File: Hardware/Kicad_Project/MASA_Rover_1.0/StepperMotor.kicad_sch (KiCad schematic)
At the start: 8 parts, among them J26 Conn_01x04_Male, J27 Conn_01x04_Male, J28 Screw_Terminal_01x01, J29 Screw_Terminal_01x01

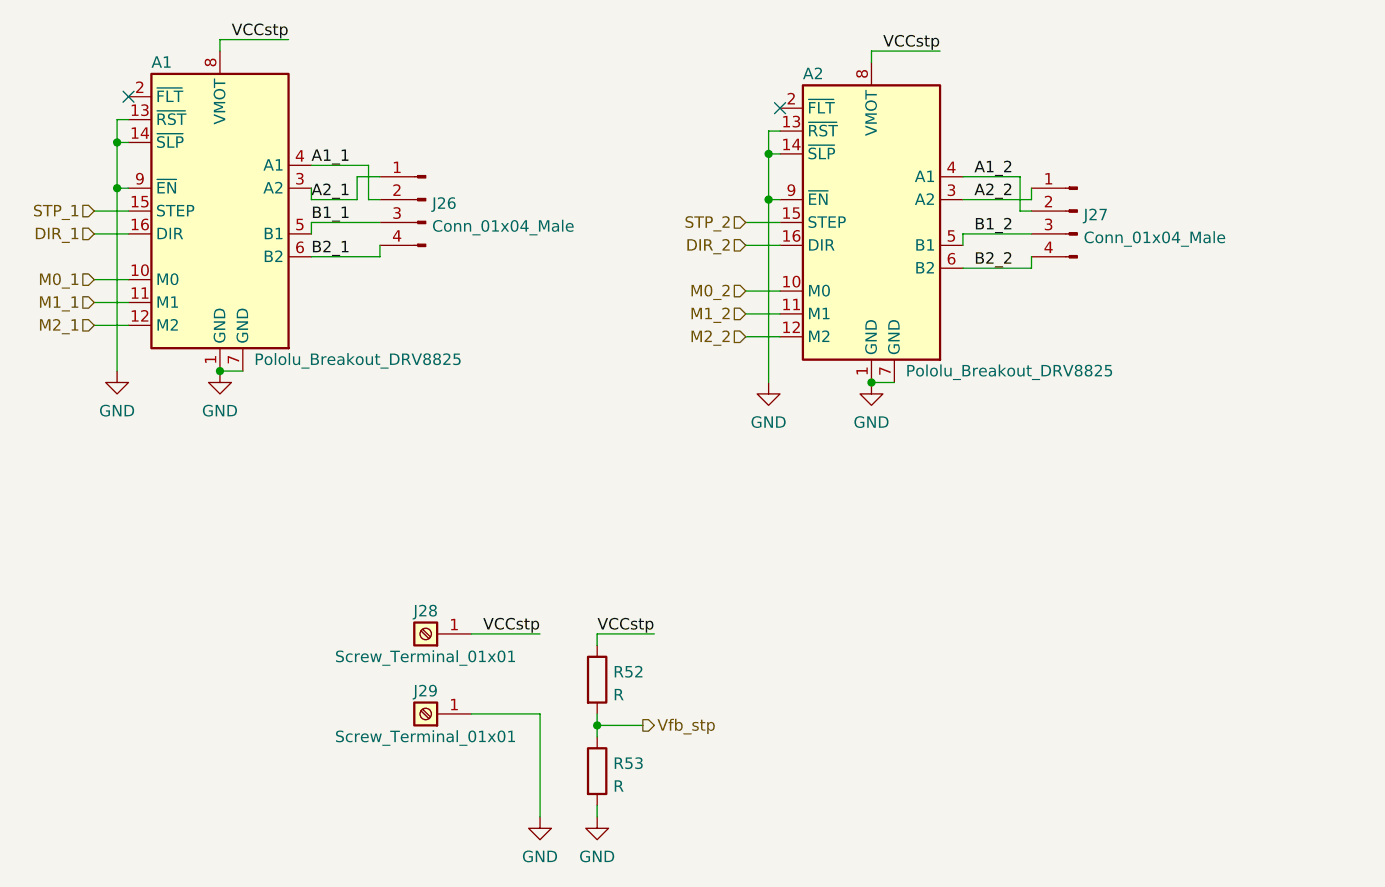
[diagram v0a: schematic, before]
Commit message: update hardware
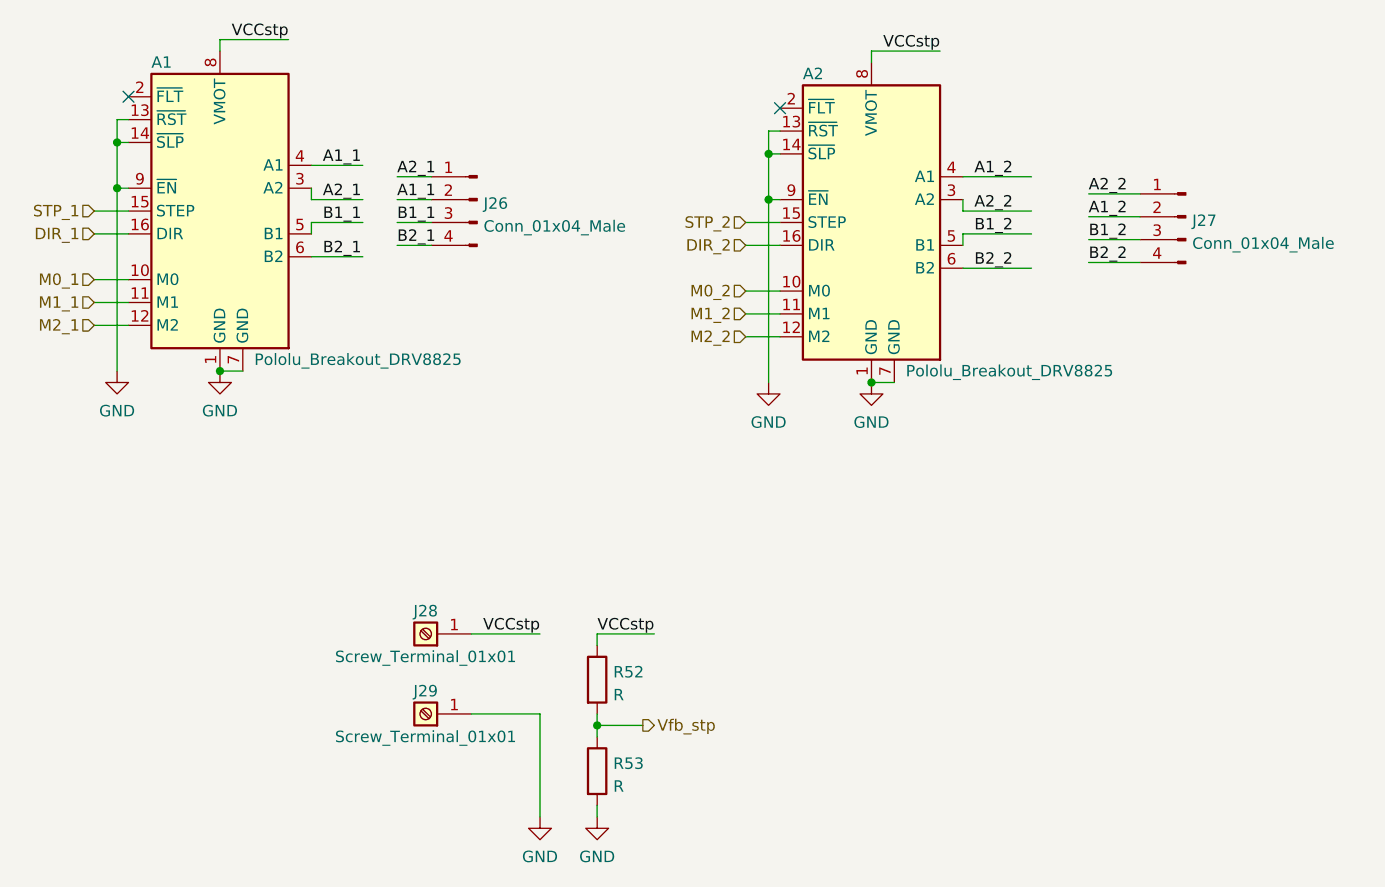
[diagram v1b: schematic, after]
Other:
- moved on the sheet: J26, J27
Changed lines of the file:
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@@
-    (stroke (width 0) (type default) (color 0 0 0 0))
-  )
-  (wire (pts (xy 97.79 81.28) (xy 97.79 85.09))
-    (stroke (width 0) (type default) (color 0 0 0 0))
-  )
-  (wire (pts (xy 96.52 85.09) (xy 96.52 82.55))
     (stroke (width 0) (type default) (color 0 0 0 0))
   )
@@
     (stroke (width 0) (type default) (color 0 0 0 0))
   )
-  (wire (pts (xy 97.79 81.28) (xy 91.44 81.28))
-    (stroke (width 0) (type default) (color 0 0 0 0))
-  )
   (wire (pts (xy 153.67 105.41) (xy 156.21 105.41))
     (stroke (width 0) (type default) (color 0 0 0 0))
@@
     (stroke (width 0) (type default) (color 0 0 0 0))
   )
-  (wire (pts (xy 171.45 92.71) (xy 171.45 91.44))
-    (stroke (width 0) (type default) (color 0 0 0 0))
-  )
-  (wire (pts (xy 97.79 85.09) (xy 99.06 85.09))
+  (wire (pts (xy 91.44 91.44) (xy 97.155 91.44))
+    (stroke (width 0) (type default) (color 0 0 0 0))
+  )
+  (wire (pts (xy 163.83 82.55) (xy 171.45 82.55))
     (stroke (width 0) (type default) (color 0 0 0 0))
   )
@@
     (stroke (width 0) (type default) (color 0 0 0 0))
   )
+  (wire (pts (xy 177.8 89.535) (xy 183.515 89.535))
+    (stroke (width 0) (type default) (color 0 0 0 0))
+  )
   (wire (pts (xy 123.19 142.24) (xy 123.19 143.51))
     (stroke (width 0) (type default) (color 0 0 0 0))
@@
     (stroke (width 0) (type default) (color 0 0 0 0))
   )
+  (wire (pts (xy 91.44 81.28) (xy 97.155 81.28))
+    (stroke (width 0) (type default) (color 0 0 0 0))
+  )
+  (wire (pts (xy 171.45 86.36) (xy 163.83 86.36))
+    (stroke (width 0) (type default) (color 0 0 0 0))
+  )
   (wire (pts (xy 67.31 96.52) (xy 71.12 96.52))
     (stroke (width 0) (type default) (color 0 0 0 0))
@@
     (stroke (width 0) (type default) (color 0 0 0 0))
   )
+  (wire (pts (xy 100.965 85.09) (xy 104.775 85.09))
+    (stroke (width 0) (type default) (color 0 0 0 0))
+  )
   (wire (pts (xy 142.24 80.01) (xy 143.51 80.01))
     (stroke (width 0) (type default) (color 0 0 0 0))
@@
     (stroke (width 0) (type default) (color 0 0 0 0))
   )
-  (wire (pts (xy 96.52 82.55) (xy 99.06 82.55))
-    (stroke (width 0) (type default) (color 0 0 0 0))
-  )
-  (wire (pts (xy 99.06 91.44) (xy 99.06 90.17))
-    (stroke (width 0) (type default) (color 0 0 0 0))
-  )
   (wire (pts (xy 88.9 67.31) (xy 81.28 67.31))
     (stroke (width 0) (type default) (color 0 0 0 0))
@@
     (stroke (width 0) (type default) (color 0 0 0 0))
   )
+  (wire (pts (xy 177.8 84.455) (xy 183.515 84.455))
+    (stroke (width 0) (type default) (color 0 0 0 0))
+  )
   (wire (pts (xy 116.84 142.24) (xy 116.84 153.67))
     (stroke (width 0) (type default) (color 0 0 0 0))
   )
+  (wire (pts (xy 100.965 87.63) (xy 104.775 87.63))
+    (stroke (width 0) (type default) (color 0 0 0 0))
+  )
   (wire (pts (xy 123.19 143.51) (xy 123.19 144.78))
     (stroke (width 0) (type default) (color 0 0 0 0))
   )
-  (wire (pts (xy 91.44 91.44) (xy 99.06 91.44))
-    (stroke (width 0) (type default) (color 0 0 0 0))
-  )
-  (wire (pts (xy 99.06 87.63) (xy 91.44 87.63))
+  (wire (pts (xy 91.44 87.63) (xy 97.155 87.63))
     (stroke (width 0) (type default) (color 0 0 0 0))
   )
@@
     (stroke (width 0) (type default) (color 0 0 0 0))
   )
-  (wire (pts (xy 91.44 85.09) (xy 96.52 85.09))
+  (wire (pts (xy 100.965 90.17) (xy 104.775 90.17))
     (stroke (width 0) (type default) (color 0 0 0 0))
   )
@@
     (stroke (width 0) (type default) (color 0 0 0 0))
   )
+  (wire (pts (xy 91.44 85.09) (xy 97.155 85.09))
+    (stroke (width 0) (type default) (color 0 0 0 0))
+  )
   (wire (pts (xy 142.24 77.47) (xy 143.51 77.47))
     (stroke (width 0) (type default) (color 0 0 0 0))
   )
-  (wire (pts (xy 170.18 86.36) (xy 171.45 86.36))
+  (wire (pts (xy 100.965 82.55) (xy 104.775 82.55))
     (stroke (width 0) (type default) (color 0 0 0 0))
   )
@@
     (stroke (width 0) (type default) (color 0 0 0 0))
   )
-  (wire (pts (xy 163.83 82.55) (xy 170.18 82.55))
-    (stroke (width 0) (type default) (color 0 0 0 0))
-  )
-  (wire (pts (xy 163.83 85.09) (xy 171.45 85.09))
+  (wire (pts (xy 163.83 86.36) (xy 163.83 85.09))
     (stroke (width 0) (type default) (color 0 0 0 0))
   )
@@
     (stroke (width 0) (type default) (color 0 0 0 0))
   )
-  (wire (pts (xy 170.18 82.55) (xy 170.18 86.36))
-    (stroke (width 0) (type default) (color 0 0 0 0))
-  )
-  (wire (pts (xy 171.45 85.09) (xy 171.45 83.82))
+  (wire (pts (xy 177.8 92.075) (xy 183.515 92.075))
+    (stroke (width 0) (type default) (color 0 0 0 0))
+  )
+  (wire (pts (xy 177.8 86.995) (xy 183.515 86.995))
     (stroke (width 0) (type default) (color 0 0 0 0))
   )
@@
     (effects (font (size 1.27 1.27)) (justify right bottom))
   )
-  (label "B1_1" (at 91.44 87.63 0)
+  (label "A1_1" (at 100.965 85.09 0)
+    (effects (font (size 1.27 1.27)) (justify left bottom))
+  )
+  (label "B1_2" (at 177.8 89.535 0)
+    (effects (font (size 1.27 1.27)) (justify left bottom))
+  )
+  (label "B1_1" (at 92.71 87.63 0)
+    (effects (font (size 1.27 1.27)) (justify left bottom))
+  )
+  (label "A2_2" (at 177.8 84.455 0)
     (effects (font (size 1.27 1.27)) (justify left bottom))
   )
@@
     (effects (font (size 1.27 1.27)) (justify right bottom))
   )
+  (label "B1_1" (at 100.965 87.63 0)
+    (effects (font (size 1.27 1.27)) (justify left bottom))
+  )
   (label "B1_2" (at 165.1 88.9 0)
     (effects (font (size 1.27 1.27)) (justify left bottom))
   )
-  (label "B2_1" (at 91.44 91.44 0)
-    (effects (font (size 1.27 1.27)) (justify left bottom))
-  )
-  (label "A1_1" (at 91.44 81.28 0)
-    (effects (font (size 1.27 1.27)) (justify left bottom))
-  )
-  (label "A2_1" (at 91.44 85.09 0)
+  (label "B2_1" (at 92.71 91.44 0)
+    (effects (font (size 1.27 1.27)) (justify left bottom))
+  )
+  (label "A1_1" (at 92.71 81.28 0)
+    (effects (font (size 1.27 1.27)) (justify left bottom))
+  )
+  (label "A2_1" (at 92.71 85.09 0)
+    (effects (font (size 1.27 1.27)) (justify left bottom))
+  )
+  (label "B2_1" (at 100.965 90.17 0)
+    (effects (font (size 1.27 1.27)) (justify left bottom))
+  )
+  (label "A2_1" (at 100.965 82.55 0)
+    (effects (font (size 1.27 1.27)) (justify left bottom))
+  )
+  (label "B2_2" (at 177.8 92.075 0)
     (effects (font (size 1.27 1.27)) (justify left bottom))
   )
@@
     (effects (font (size 1.27 1.27)) (justify right bottom))
   )
+  (label "A1_2" (at 177.8 86.995 0)
+    (effects (font (size 1.27 1.27)) (justify left bottom))
+  )
   (label "VCCstp" (at 116.84 133.35 180)
     (effects (font (size 1.27 1.27)) (justify right bottom))
   )
-  (label "A2_2" (at 165.1 85.09 0)
+  (label "A2_2" (at 165.1 86.36 0)
     (effects (font (size 1.27 1.27)) (justify left bottom))
   )
@@
     (pin "1")
   )
-  (symbol (lib_id "Connector:Conn_01x04_Male") (at 104.14 85.09 0) (mirror y) (unit 1)
-    (in_bom yes) (on_board yes) (fields_autoplaced)
-    (property "Reference" "J26" (id 0) (at 104.8512 85.5253 0)
+  (symbol (lib_id "Connector:Conn_01x04_Male") (at 109.855 85.09 0) (mirror y) (unit 1)
+    (in_bom yes) (on_board yes) (fields_autoplaced)
+    (property "Reference" "J26" (id 0) (at 110.5662 85.5253 0)
       (effects (font (size 1.27 1.27)) (justify right))
     )
-    (property "Value" "Conn_01x04_Male" (id 1) (at 104.8512 88.0622 0)
+    (property "Value" "Conn_01x04_Male" (id 1) (at 110.5662 88.0622 0)
       (effects (font (size 1.27 1.27)) (justify right))
     )
-    (property "Footprint" "Connector_PinHeader_2.54mm:PinHeader_1x04_P2.54mm_Vertical" (id 2) (at 104.14 85.09 0)
-      (effects (font (size 1.27 1.27)) hide)
-    )
-    (property "Datasheet" "~" (id 3) (at 104.14 85.09 0)
+    (property "Footprint" "Connector_PinHeader_2.54mm:PinHeader_1x04_P2.54mm_Vertical" (id 2) (at 109.855 85.09 0)
+      (effects (font (size 1.27 1.27)) hide)
+    )
+    (property "Datasheet" "~" (id 3) (at 109.855 85.09 0)
       (effects (font (size 1.27 1.27)) hide)
     )
@@
     (pin "1")
   )
-  (symbol (lib_id "Connector:Conn_01x04_Male") (at 176.53 86.36 0) (mirror y) (unit 1)
-    (in_bom yes) (on_board yes) (fields_autoplaced)
-    (property "Reference" "J27" (id 0) (at 177.2412 86.7953 0)
+  (symbol (lib_id "Connector:Conn_01x04_Male") (at 188.595 86.995 0) (mirror y) (unit 1)
+    (in_bom yes) (on_board yes) (fields_autoplaced)
+    (property "Reference" "J27" (id 0) (at 189.3062 87.4303 0)
       (effects (font (size 1.27 1.27)) (justify right))
     )
-    (property "Value" "Conn_01x04_Male" (id 1) (at 177.2412 89.3322 0)
+    (property "Value" "Conn_01x04_Male" (id 1) (at 189.3062 89.9672 0)
       (effects (font (size 1.27 1.27)) (justify right))
     )
-    (property "Footprint" "Connector_PinHeader_2.54mm:PinHeader_1x04_P2.54mm_Vertical" (id 2) (at 176.53 86.36 0)
-      (effects (font (size 1.27 1.27)) hide)
-    )
-    (property "Datasheet" "~" (id 3) (at 176.53 86.36 0)
-      (effects (font (size 1.27 1.27)) hide)
-    )
+    (property "Footprint" "Connector_PinHeader_2.54mm:PinHeader_1x04_P2.54mm_Vertical" (id 2) (at 188.595 86.995 0)
+      (effects (font (size 1.27 1.27)) hide)
+    )
+    (property "Datasheet" "~" (id 3) (at 188.595 86.995 0)
+      (effects (font (size 1.27 1.27)) hide)
+    )
